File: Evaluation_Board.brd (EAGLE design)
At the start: 60.9 x 39.4 mm, 38 parts, among them IC1 MEGA32-A, IC2 FT232RL, IC3 317EMP, J1 DCJ0202, Q1 16 MHz

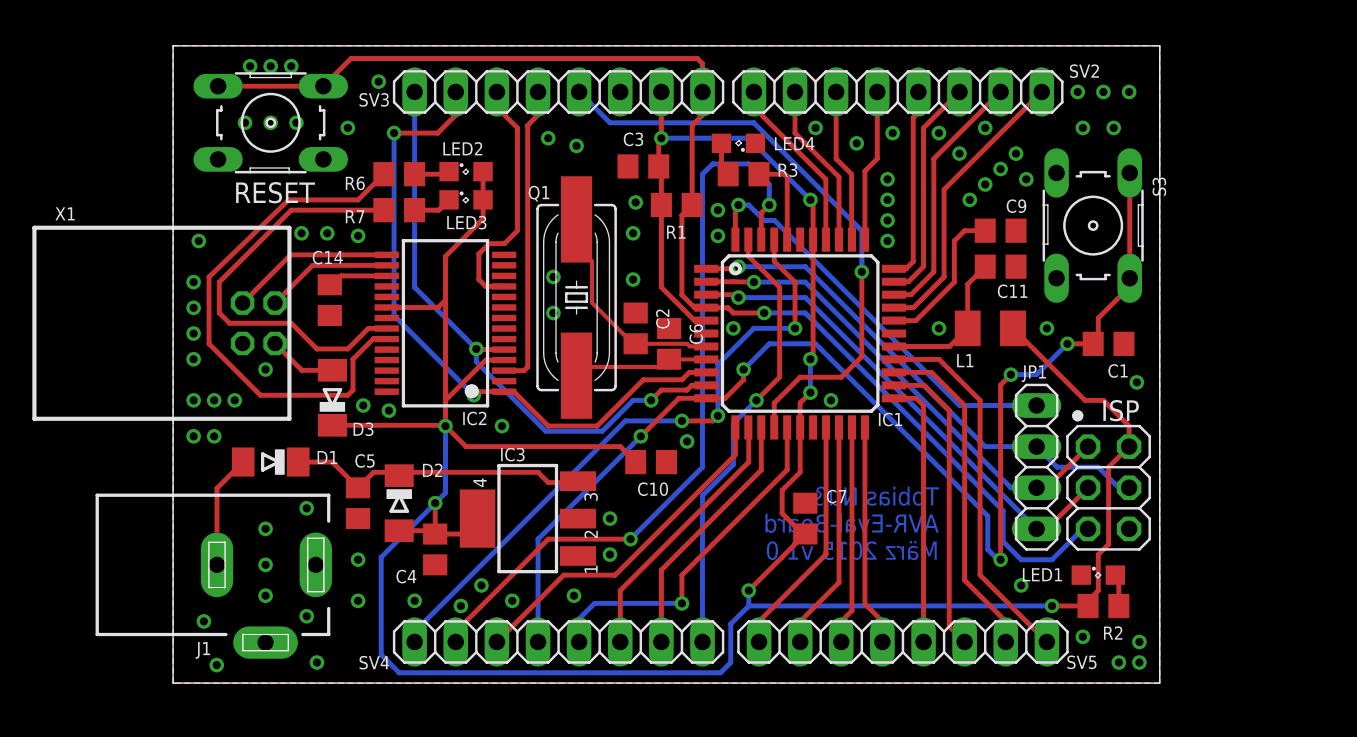
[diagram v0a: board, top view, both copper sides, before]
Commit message: Test mit einem neuen Branch namens edit.
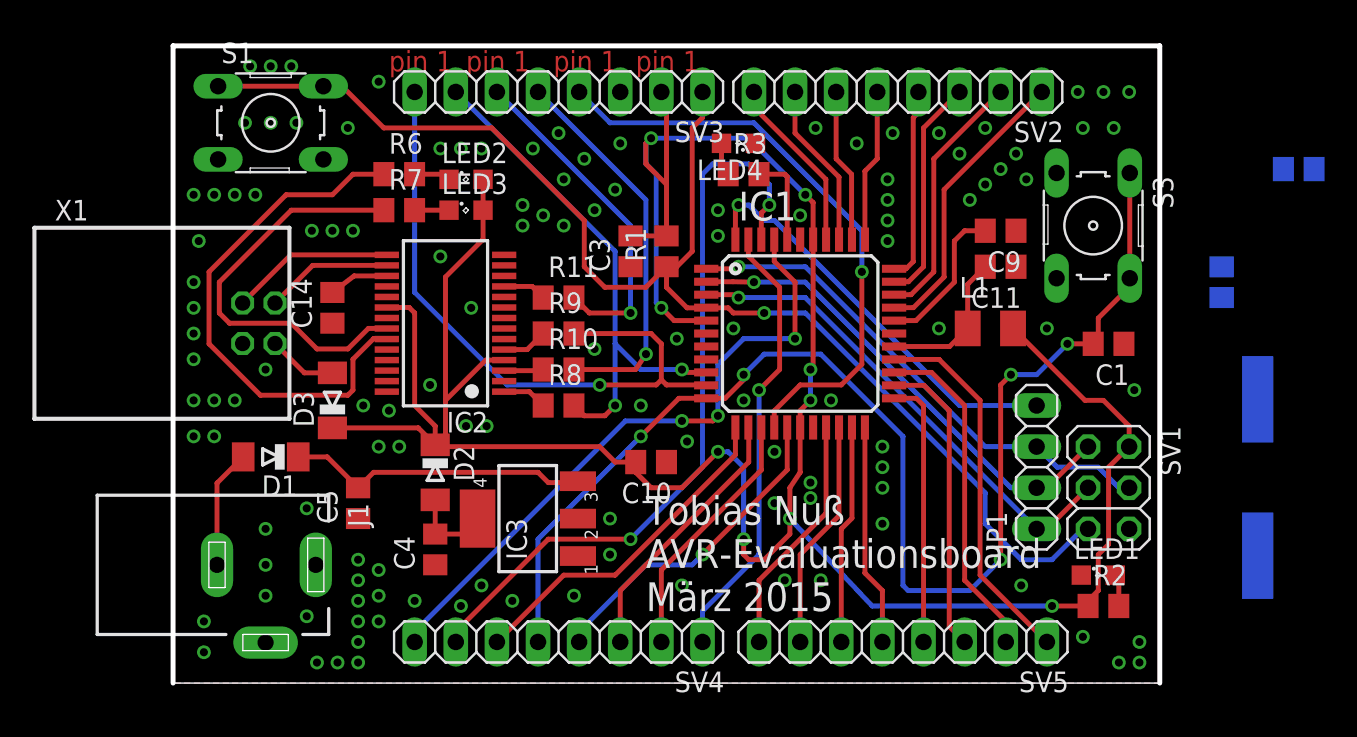
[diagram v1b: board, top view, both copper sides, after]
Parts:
- removed C7: 100n, rcl:C0805
- added R10, R11, R8, R9: 1k, rcl:R0805
- C2, C6: value 12p -> 100n
- Q1: value 16 MHz -> (none)
- moved Q1 43.5 mm to (67.0, 12.7), flipped to the bottom
- moved C6 40.4 mm to (69.5, 31.8), flipped to the bottom, turned to 180 degrees
- moved C2 36.3 mm to (64.8, 24.8), flipped to the bottom
- moved C3 5.30 mm to (28.3, 26.7), turned to 90 degrees
- moved D2 2.93 mm to (16.2, 13.0)
- moved R1 2.93 mm to (30.5, 26.7), turned to 90 degrees
- moved LED3 0.63 mm to (18.1, 29.2)
- moved C14 0.50 mm to (9.84, 23.2)
- moved LED2 0.48 mm to (18.1, 31.1)
- moved D1 0.32 mm to (6.03, 14.0)
- moved D3 0.16 mm to (9.84, 17.5)
- renumbered ISP to SV1, RESET to S1
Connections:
- removed net N$17: C2.2, IC1.7, Q1.2
- removed net N$25: C6.2, IC1.8, Q1.1
- new net N$2: C4.2, D2.A, IC3.4
- new net N$21: IC2.1, R8.1
- new net N$22: IC2.5, R9.1
- new net N$23: IC2.3, R10.1
- new net N$24: IC2.11, R11.1
- net +5V: now also D2.C; no longer C4.2, C7.2, D2.A, IC3.4
- net CTS: now also R11.2; no longer IC2.11
- net GND: no longer C2.1, C6.1, C7.1
- net NETZ: no longer D2.C
- net RTS: now also R10.2; no longer IC2.3
- net RX_USB: now also R8.2; no longer IC2.1
- net TX_USB: now also R9.2; no longer IC2.5
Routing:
- net +5V: track 191.8 -> 174.9 mm, vias 8 -> 9
- net N$17: track 13.9 -> 0.00 mm
- net N$25: track 8.82 -> 0.00 mm
- net RX_USB: track 40.6 -> 32.9 mm
- net CTS: track 15.4 -> 21.0 mm, vias 0 -> 1
- net N$2: track 0.00 -> 5.12 mm
- net RTS: track 18.8 -> 23.9 mm, vias 0 -> 1
- net PD2_INT0: track 76.1 -> 81.1 mm
- net RESET: track 79.3 -> 83.3 mm
- net TX_USB: track 37.4 -> 40.9 mm, vias 2 -> 1
- net N$22: track 0.00 -> 2.82 mm
- net N$21: track 0.00 -> 2.76 mm
- net N$24: track 0.00 -> 2.69 mm
- net N$23: track 0.00 -> 2.44 mm
- net OC2: track 21.7 -> 20.2 mm
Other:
- board text added: "Tobias Nuß AVR-Evaluationsboard März 2015"
- board text added: "pin 1"
- board text removed: "Tobias Nuß AVR-Eval-Board März 2015 v1.0"
